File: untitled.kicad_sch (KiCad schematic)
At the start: 50 parts, among them J1 Conn_01x04_Pin, J10 Conn_01x03_Pin, J2 USB_B_Micro, J3 Conn_01x02_Pin, J4 Conn_01x02_Pin, J6 Screw_Terminal_01x02, J9 Screw_Terminal_01x02, U1 STM32F767ZITx, U5 AT24C256, U8 AMS1117-3.3, U9 AMS1117-3.3, Y1 16MHz

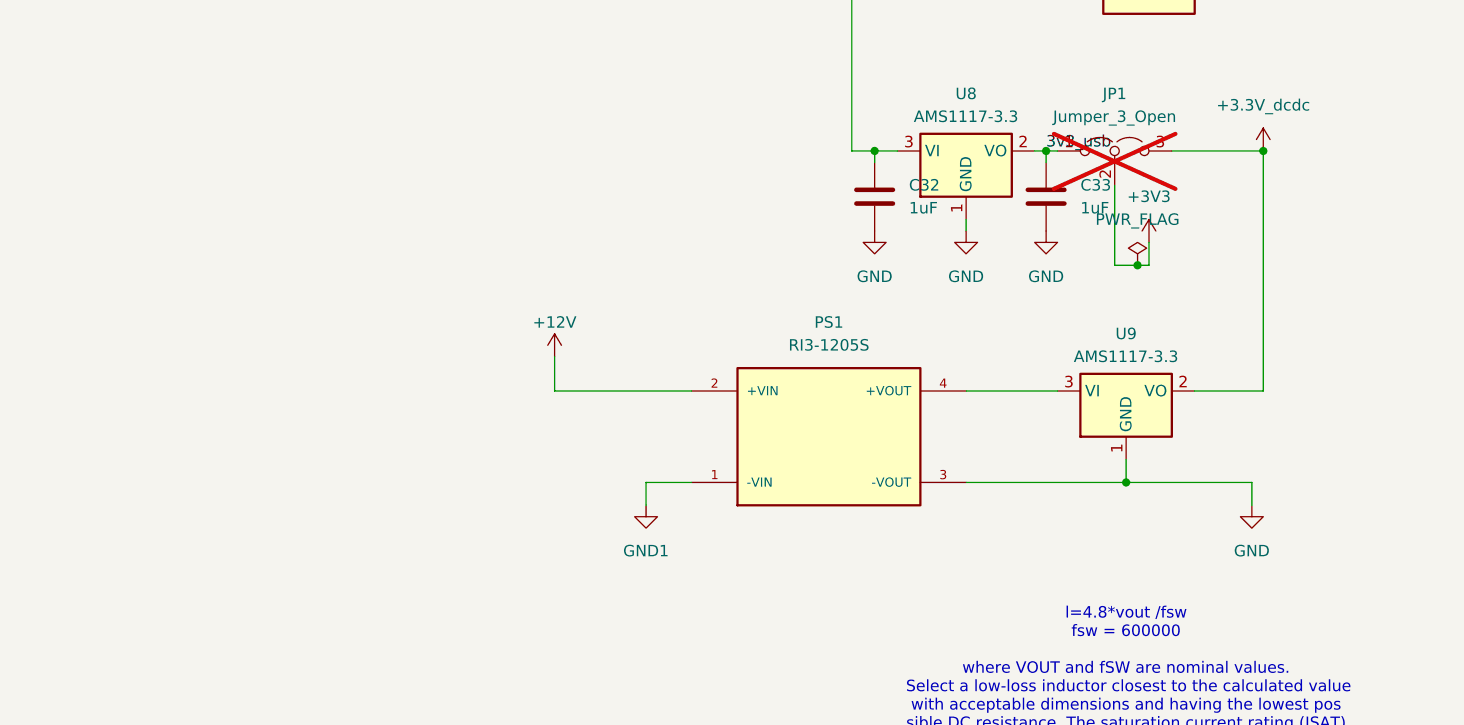
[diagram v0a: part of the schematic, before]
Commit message: Autosave
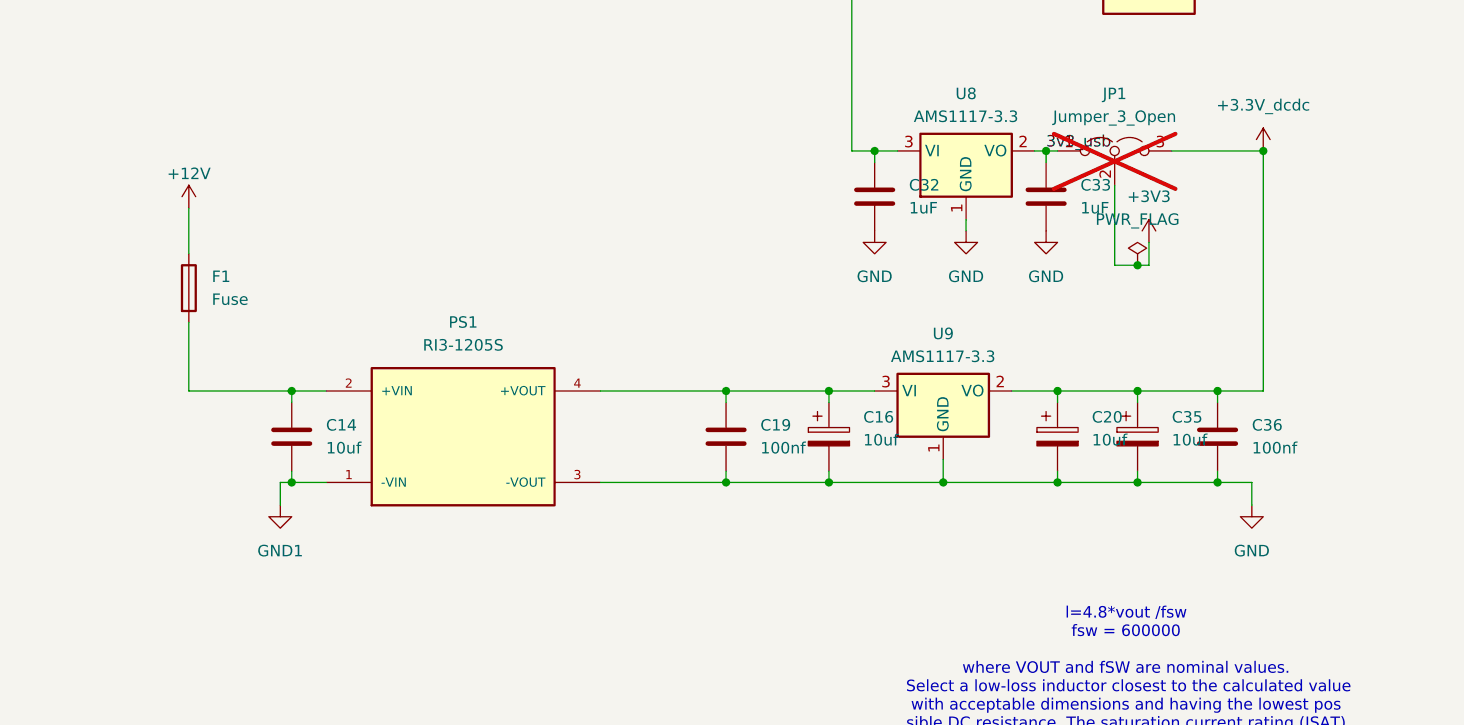
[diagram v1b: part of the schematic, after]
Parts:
- added C14: 10uf, Capacitor_SMD:C_0805_2012Metric, symbol Device:C
- added C16, C20, C35: 10uf, Capacitor_Tantalum_SMD:CP_EIA-3216-18_Kemet-A, symbol Device:C_Polarized
- added C19, C36: 100nf, Capacitor_SMD:C_0402_1005Metric, symbol Device:C
- added F1: Fuse, Fuse:Fuse_0603_1608Metric_Pad1.05x0.95mm_HandSolder, symbol Device:Fuse
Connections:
- net +12V: now also F1.1; no longer PS1.2 (+VIN)
- net +3.3V_dcdc: now also C20.1, C35.1, C36.1
- net GND: now also C16.2, C19.2, C20.2, C35.2, C36.2
- net GND1: now also C14.2
- net at PS1.4 (+VOUT), U9.3 (VI): now also C16.1, C19.1
- new net: C14.1, F1.2, PS1.2 (+VIN)
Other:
- moved on the sheet: PS1, U9
